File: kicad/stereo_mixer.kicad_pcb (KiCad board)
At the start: 2 copper layers, 70 x 75 mm, 67 parts, among them J101 DC In, J102 Output, J103 Input CH1, J104 Input CH2, J105 Input CH3, J106 Input CH4/5, SW101 Power, U101 LM317L_SO8, U301 LM358, U302 LM358, U401 LM358, U402 LM358, U403 LM358

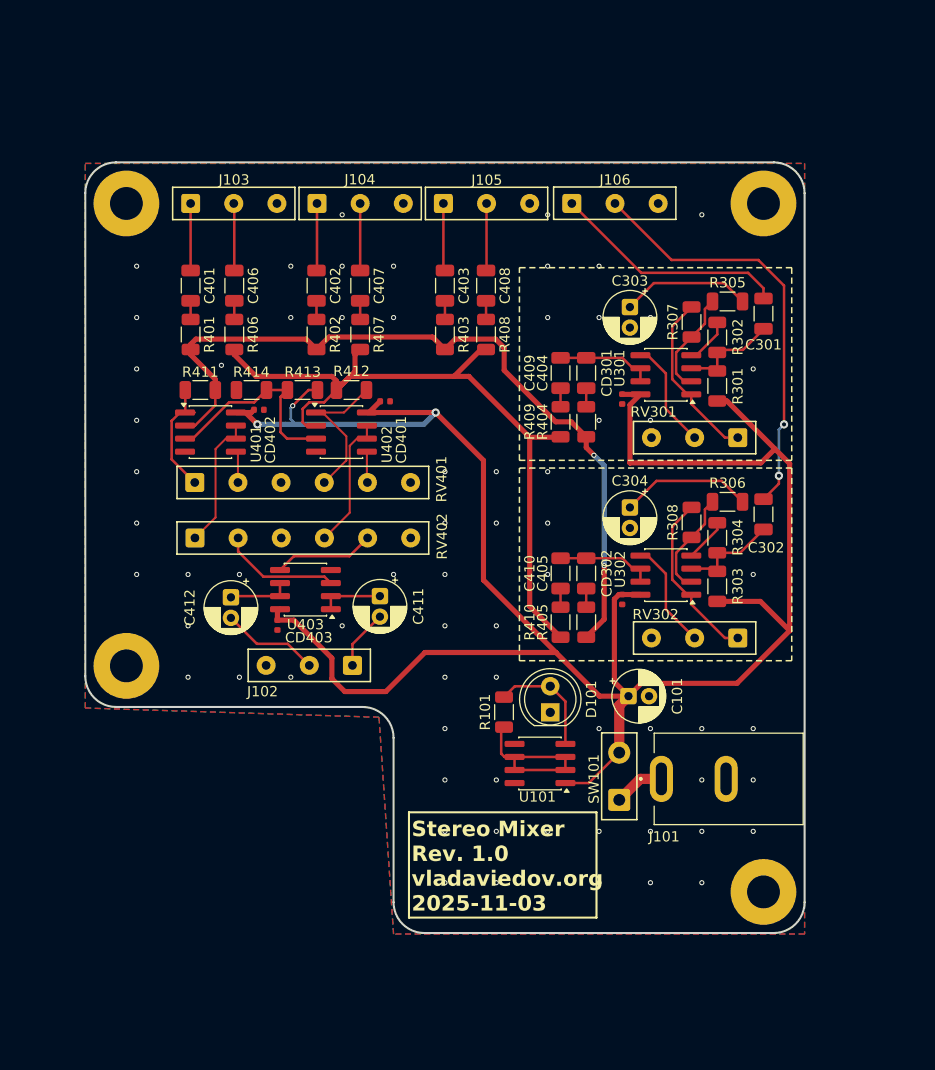
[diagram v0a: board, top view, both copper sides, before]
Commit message: redesign pcb for 1.1
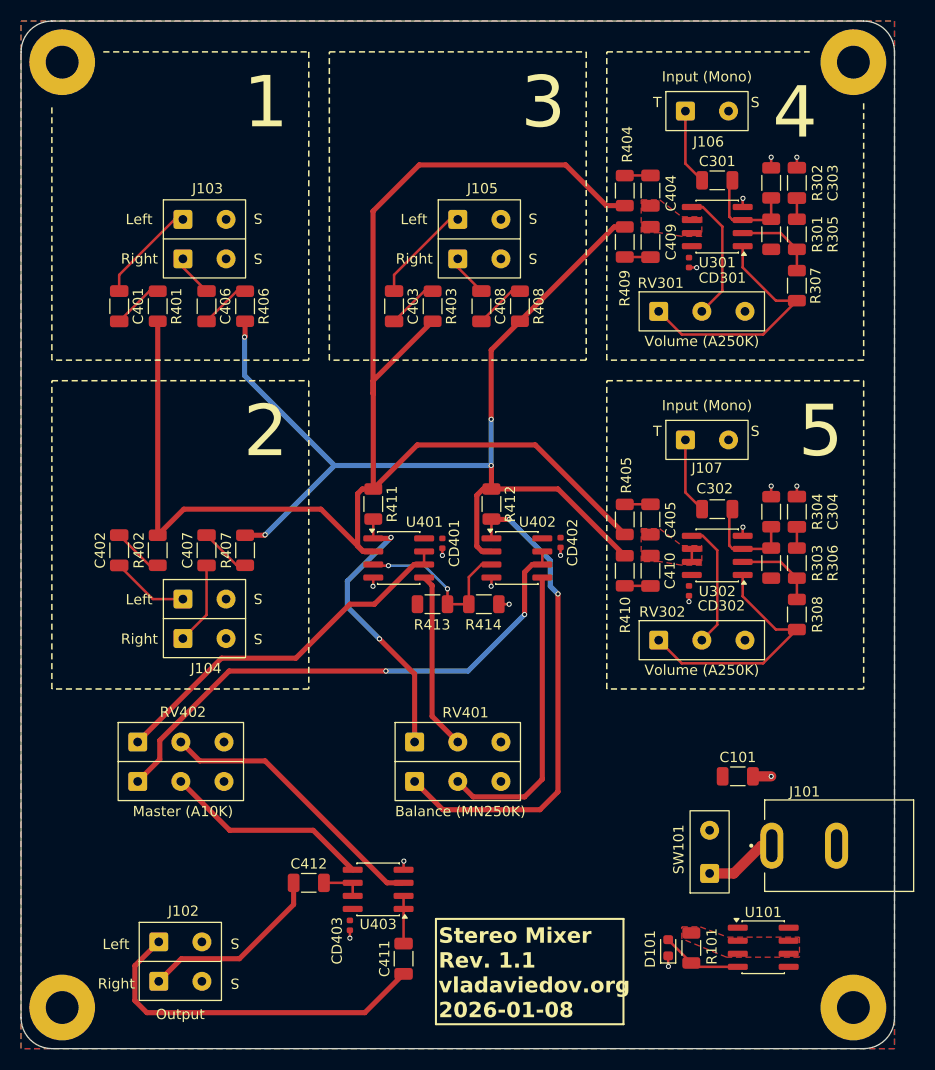
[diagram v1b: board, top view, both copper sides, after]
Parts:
- added J107: Input CH5, Custom:ChassisMount_Wire-0.25sqmm_1x02_P4.2mm_D0.65mm_OD1.7mm, F.Cu at (136.2, 70.3)
- added REF**: KiCad-Logo2_12mm_SilkScreen, Symbol:KiCad-Logo2_12mm_SilkScreen, B.Cu at (113.9, 117.6)
- added REF**: Polarity_Center_Positive_6mm_SilkScreen, Symbol:Polarity_Center_Positive_6mm_SilkScreen, B.Cu at (142.2, 101.6)
- C101, C411, C412: footprint Capacitor_THT:CP_Radial_D5.0mm_P2.00mm -> Capacitor_SMD:C_1206_3216Metric
- C303, C304: value 4.7uF -> 10uF; footprint Capacitor_THT:CP_Radial_D5.0mm_P2.00mm -> Capacitor_SMD:C_1206_3216Metric
- D101: value LED -> Green; footprint LED_THT:LED_D5.0mm -> LED_SMD:LED_0603_1608Metric
- J102, J103, J104, J105: footprint Connector_Wire:SolderWire-0.25sqmm_1x03_P4.2mm_D0.65mm_OD1.7mm -> Custom:ChassisMount_Wire-0.25sqmm_2x02_P4.2mm_D0.65mm_OD1.7mm
- J106: value Input CH4/5 -> Input CH4; footprint Connector_Wire:SolderWire-0.25sqmm_1x03_P4.2mm_D0.65mm_OD1.7mm -> Custom:ChassisMount_Wire-0.25sqmm_1x02_P4.2mm_D0.65mm_OD1.7mm
- RV301, RV302: footprint Connector_Wire:SolderWire-0.25sqmm_1x03_P4.2mm_D0.65mm_OD1.7mm -> Custom:ChassisMount_Wire-0.25sqmm_1x03_P4.2mm_D0.65mm_OD1.7mm
- RV401, RV402: footprint Connector_Wire:SolderWire-0.25sqmm_1x06_P4.2mm_D0.65mm_OD1.7mm -> Custom:ChassisMount_Wire-0.25sqmm_2x03_P4.2mm_D0.65mm_OD1.7mm
- SW101: value Power -> SPST; footprint Connector_Wire:SolderWire-0.5sqmm_1x02_P4.6mm_D0.9mm_OD2.1mm -> Custom:ChassisMount_Wire-0.25sqmm_1x02_P4.2mm_D0.65mm_OD1.7mm
- moved H104 78.2 mm to (152.5, 125.5)
- moved H103 69.2 mm to (75.5, 125.5)
- moved J104 40.7 mm to (87.2, 85.8)
- moved C411 35.4 mm to (108.7, 120.8), turned to 90 degrees
- moved RV401 33.1 mm to (109.8, 99.7)
- moved J102 32.9 mm to (84.9, 119.1), turned to 0 degrees
- moved C402 32.1 mm to (81.0, 81.0), turned to 90 degrees
- moved CD402 32.1 mm to (124.0, 80.2), turned to -90 degrees
- moved R414 30.8 mm to (116.5, 86.2), turned to 0 degrees
- moved CD403 30.1 mm to (103.5, 117.5)
- moved U403 30.0 mm to (106.2, 114.0)
- moved C407 29.8 mm to (89.5, 81.0), turned to 90 degrees
- moved R101 29.3 mm to (136.7, 119.7), turned to -90 degrees
- moved C412 28.8 mm to (99.5, 113.4), turned to 0 degrees
- moved U101 28.1 mm to (143.7, 119.6), turned to 0 degrees
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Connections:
- C411 pad 1: Net-(U403A--) -> /OUT.L
- C411 pad 2: /OUT.L -> Net-(U403A--)
- C412 pad 1: Net-(U403B--) -> /OUT.R
- C412 pad 2: /OUT.R -> Net-(U403B--)
- J102 pad 2: /OUT.R -> GND
- J102 pad 3: GND -> /OUT.R
- J103 pad 2: /CH1.R -> GND
- J103 pad 3: GND -> /CH1.R
- J104 pad 2: /CH2.R -> GND
- J104 pad 3: GND -> /CH2.R
- J105 pad 2: /CH3.R -> GND
- J105 pad 3: GND -> /CH3.R
- J106 pad 2: /CH5 -> GND
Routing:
- net VCC: track 209.0 -> 0.00 mm, vias 3 -> 0
- net Net-(U401A--): track 77.4 -> 146.8 mm, vias 2 -> 0
- net Net-(U402B--): track 13.2 -> 52.9 mm, vias 0 -> 2
- net /CH5: track 41.4 -> 7.41 mm, vias 2 -> 0
- net Net-(R412-Pad2): track 15.1 -> 47.9 mm, vias 0 -> 2
- net /OUT.L: track 5.85 -> 34.9 mm
- net Net-(U402A--): track 73.8 -> 100.3 mm, vias 0 -> 4
- net Net-(U402B-+): track 3.02 -> 29.2 mm
- net Net-(U401B--): track 13.2 -> 36.3 mm
- net Net-(R101-Pad1): track 16.6 -> 0.00 mm
- net Net-(R411-Pad2): track 11.7 -> 28.1 mm, vias 0 -> 2
- net Net-(U403A-+): track 11.6 -> 27.4 mm
- net /CH4: track 23.1 -> 7.41 mm
- net Net-(U401B-+): track 3.08 -> 17.4 mm
- net Net-(C304-Pad1): track 12.9 -> 2.06 mm
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- added copper zone on F.Cu, net /Mixers/CH4.L
- added copper zone on F.Cu, net /Mixers/CH5.L
- added copper zone on F.Cu, net Net-(R101-Pad1)
- added copper zone on F.Cu, net VCC
- removed copper zone on F.Cu, net GND
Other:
- board size 70 x 75 mm -> 85 x 100 mm
- board text added: "1"
- board text added: "2"
- board text added: "3"
- board text added: "4"
- board text added: "5"
- board text added: "Balance (MN250K)"
- board text added: "Input (Mono)"
- board text added: "Left"
- board text added: "Master (A10K)"
- board text added: "Output"
- board text added: "Right"
- board text added: "S"
- board text added: "T"
- board text added: "Volume (A250K)"
- board text removed: "{ "ViaStitching": "0.2", "GND": { "HSpacing": "5", "VSpacing": "5", "HOffset": "0", "VOffset": "0", "Clearance": "0.5", "Randomize": false } }"
